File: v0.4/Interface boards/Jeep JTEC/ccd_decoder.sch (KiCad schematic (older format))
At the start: 10 parts, among them Q1 AO3400, Q2 IRF7317

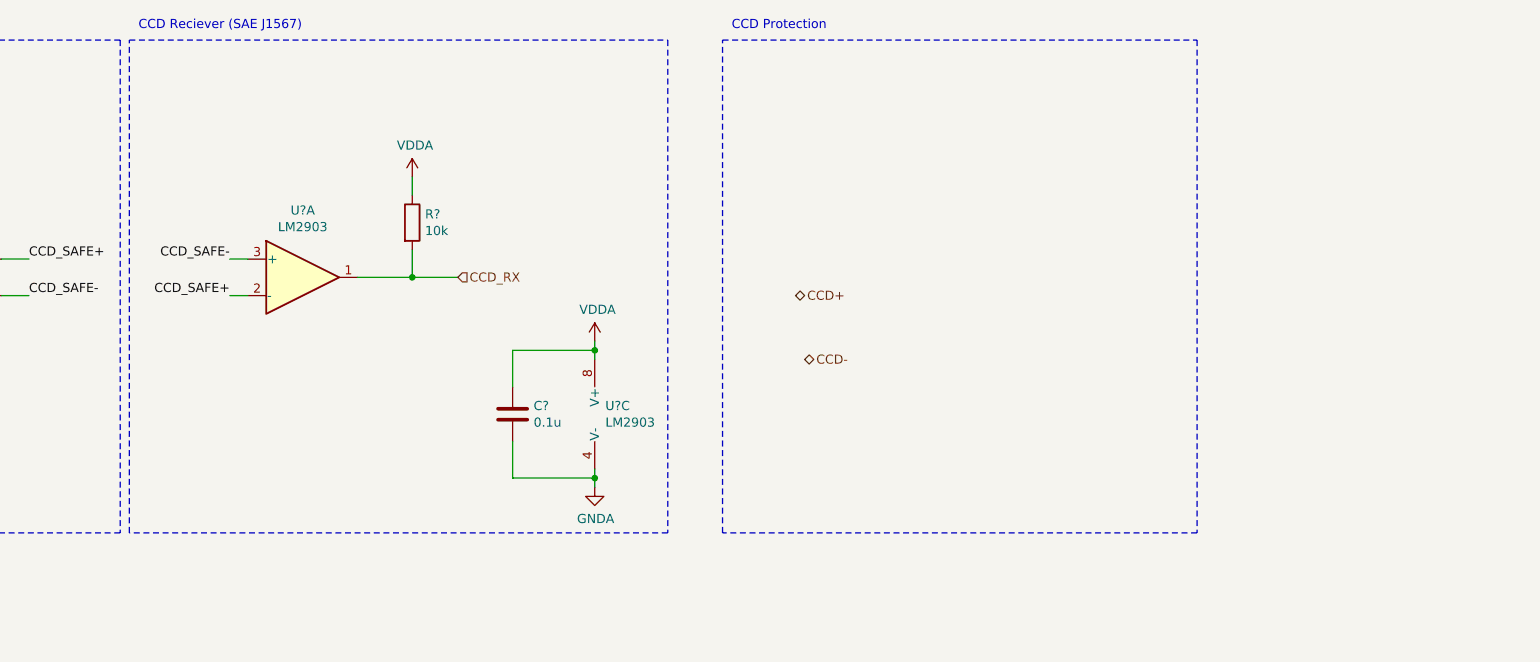
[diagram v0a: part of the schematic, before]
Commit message: Draw Jeep igniters and cruise control drivers
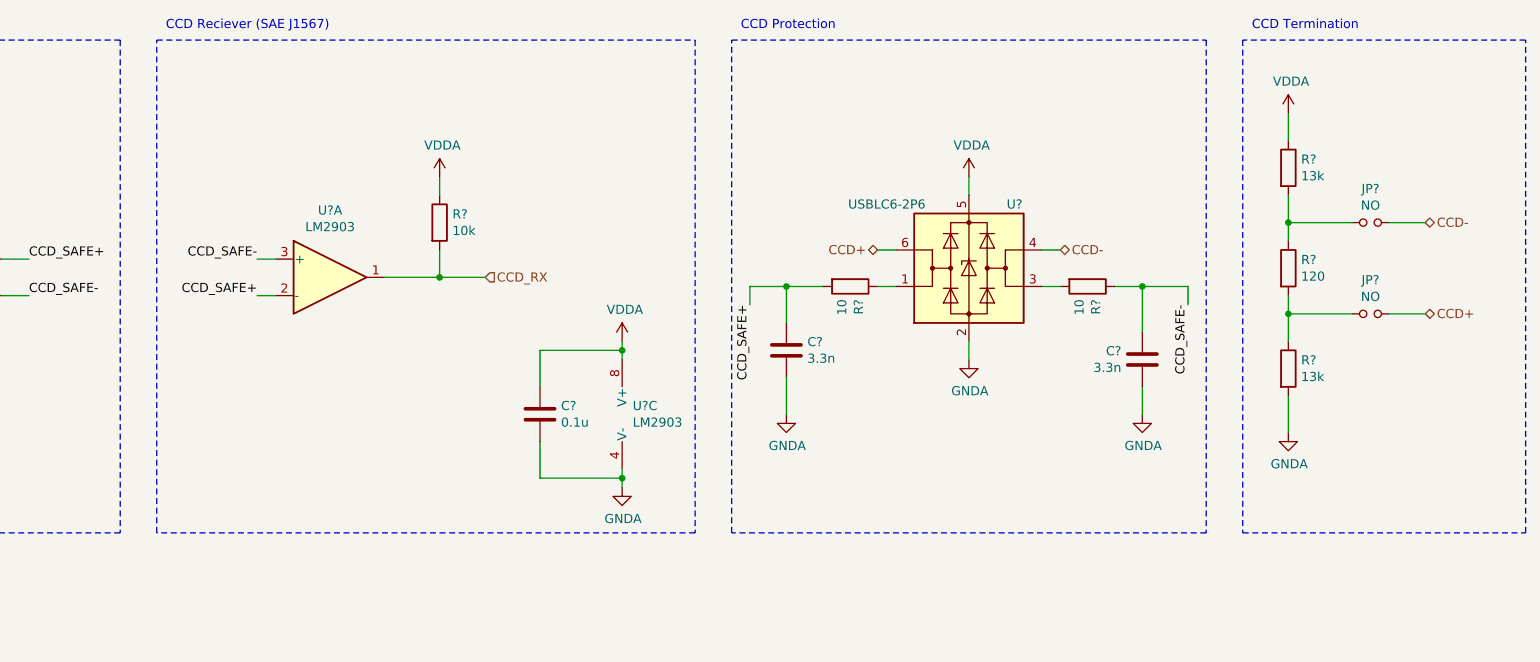
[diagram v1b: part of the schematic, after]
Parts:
- added C? (x2): 3.3n, symbol Device:C
- added JP? (x2): NO, symbol Device:Jumper_NO_Small
- added R? (x2): 10, symbol Device:R
- added R? (x2): 13k, symbol Device:R
- added R?: 120, symbol Device:R
- added U?: USBLC6-2P6, Package_TO_SOT_SMD:SOT-666, symbol Power_Protection:USBLC6-2P6
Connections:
- net CCD+: now also JP?.2, U?.6 (I/O1)
- net CCD-: now also JP?.2, U?.4 (I/O2)
- net CCD_SAFE+: now also C?.1, R?.2
- net CCD_SAFE-: now also C?.1, R?.1
- net GNDA: now also C?.2, C?.2, R?.2, U?.2 (GND)
- net VDDA: now also R?.1, U?.5 (VBUS)
- new net: R?.1, U?.1 (I/O1)
- new net: R?.2, U?.3 (I/O2)
- new net: JP?.1, R?.1, R?.2 (x2)
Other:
- note added: "CCD Termination"
- moved on the sheet: C?, R?, U?A, U?C
